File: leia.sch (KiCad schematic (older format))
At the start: 31 parts, among them J1101 TARGET_PWR, J1102 TARGET_GND, J1103 TARGET_EXT_PWR, J1112 TARGET_SHUNT, J6 EXT_READER_VCC, U1001 FOD8001, U520 FOD8012A

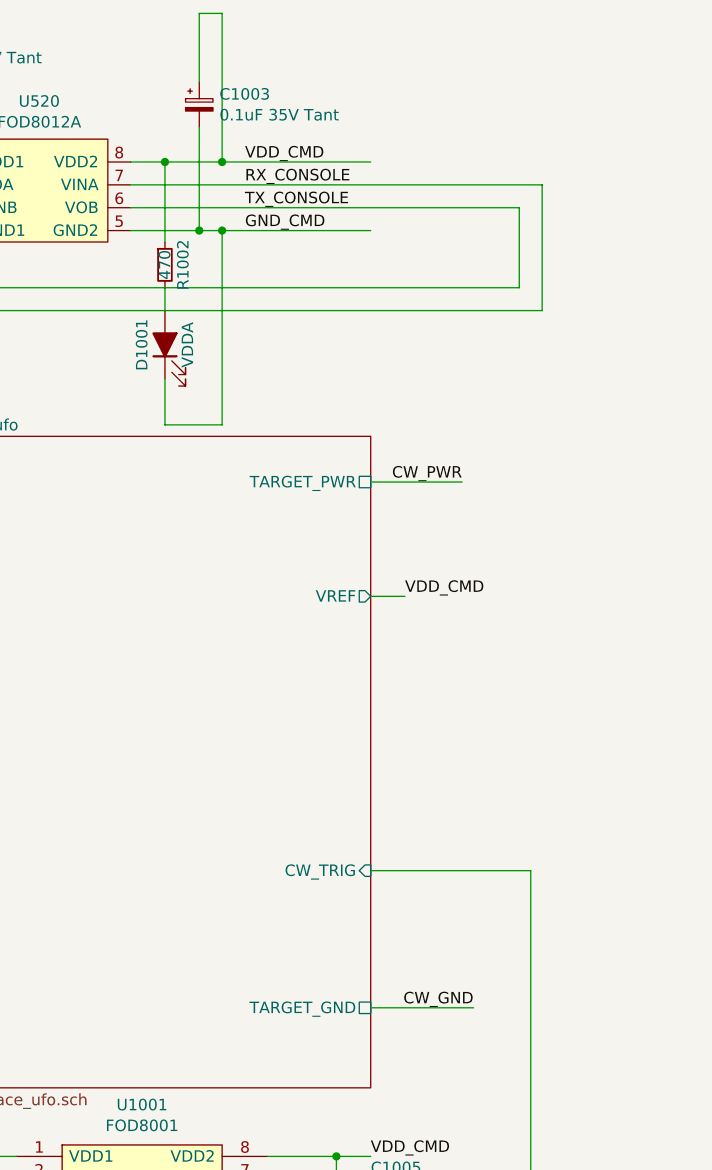
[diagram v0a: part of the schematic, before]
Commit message: [Fix] General cleanup before production
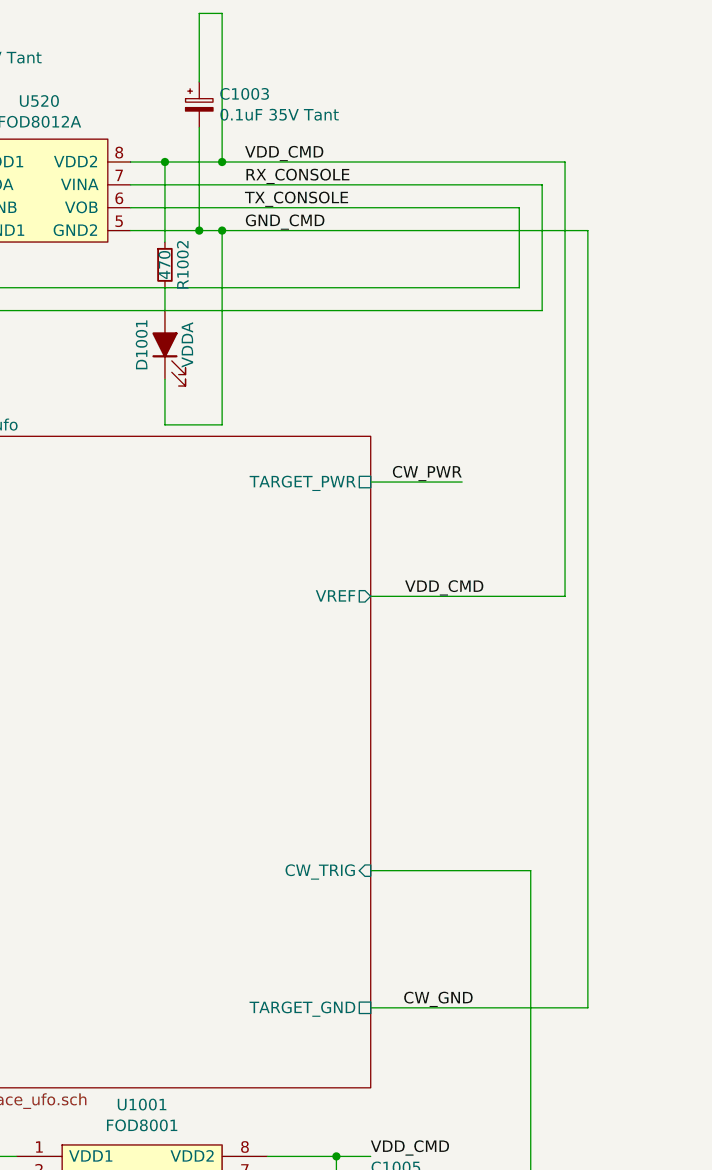
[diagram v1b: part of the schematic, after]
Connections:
- wire segments 150 -> 152
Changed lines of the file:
@@
 Text Label 15200 7200 2    50   ~ 0
 CW_GND
-Wire Wire Line
-	14750 7200 15200 7200
 Connection ~ 7250 10100
 Text Label 6700 4100 2    50   ~ 0
@@
 Wire Wire Line
 	14000 3800 14100 3800
-Wire Wire Line
-	14100 3500 14750 3500
 Wire Wire Line
 	11900 4950 11900 3600
@@
 	14100 4650 14100 3800
 Connection ~ 14100 3800
-Wire Wire Line
-	14100 3800 14750 3800
 Text Label 14200 3500 0    50   ~ 0
 VDD_CMD
@@
 Text Label 14900 5400 0    50   ~ 0
 VDD_CMD
-Wire Wire Line
-	14750 5400 14900 5400
 Text Label 14750 8150 0    50   ~ 0
 GND_CMD
@@
 Wire Wire Line
 	12700 4050 15400 4050
+Wire Wire Line
+	14100 3500 15600 3500
+Wire Wire Line
+	14750 5400 15600 5400
+Wire Wire Line
+	15600 3500 15600 5400
+Wire Wire Line
+	15700 7200 15700 3800
+Wire Wire Line
+	14100 3800 15700 3800
+Wire Wire Line
+	14750 7200 15700 7200
 $EndSCHEMATC
